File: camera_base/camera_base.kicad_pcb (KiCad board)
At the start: 2 copper layers, 80 x 80 mm, 15 parts, among them J1 Raspberry_Pi_4, J2 Conn_02x06_Odd_Even, SW1 SW_Push_Dual, SW2 SW_Push_Dual, SW3 SW_Push_Dual, SW4 SW_Push_Dual, SW5 SW_Push_Dual

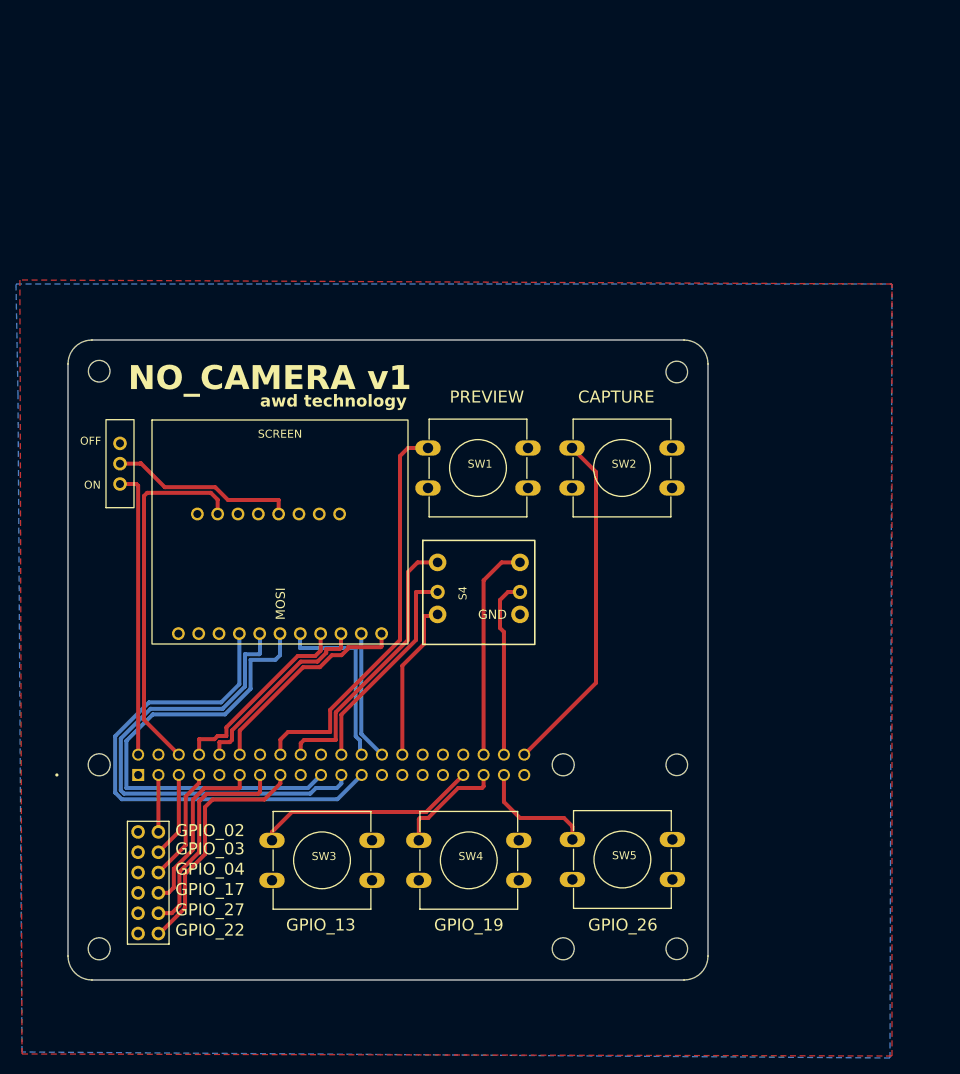
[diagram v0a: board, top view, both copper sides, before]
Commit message: update
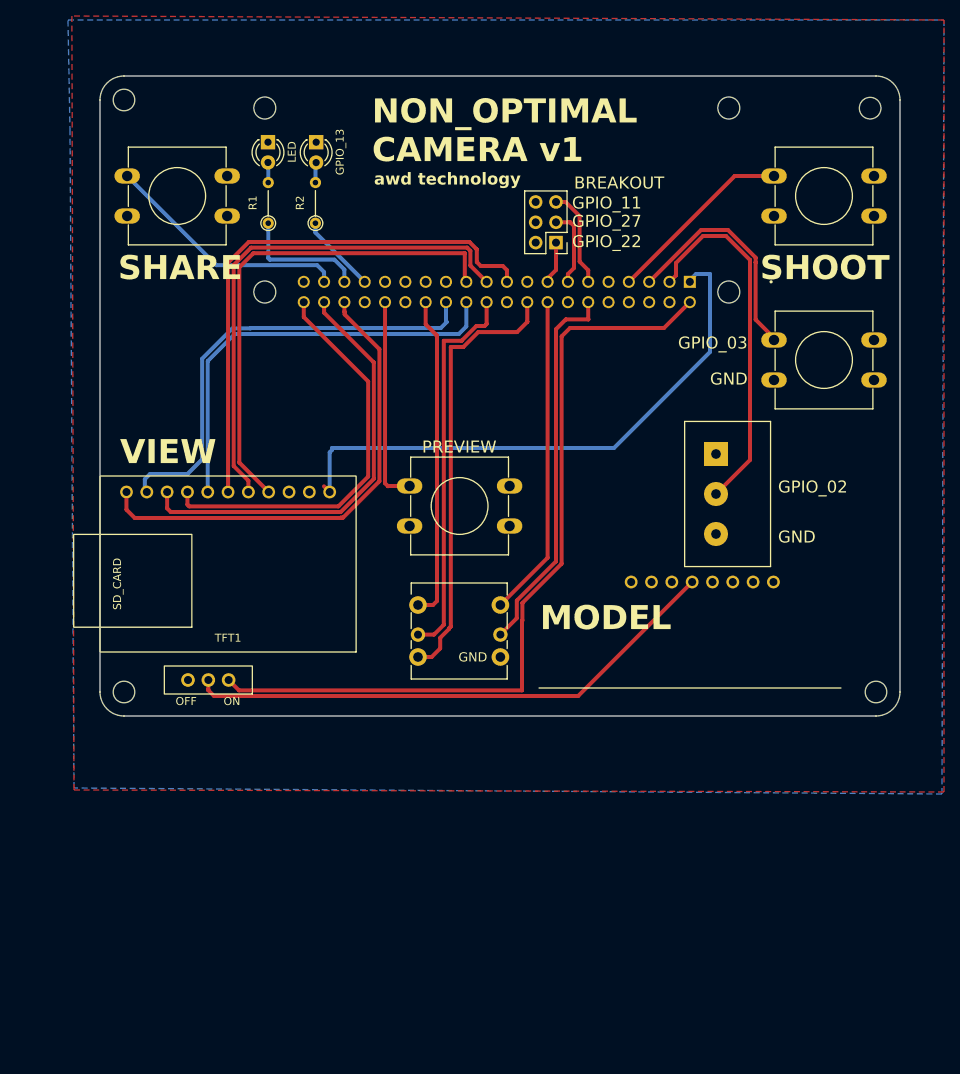
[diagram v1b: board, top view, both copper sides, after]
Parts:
- removed SW4: SW_Push_Dual, camera_base:PUSH_BUTTON_12mm
- added D1: LED, LED_THT:LED_D3.0mm, F.Cu at (81.0, 68.3)
- added D2: LED, LED_THT:LED_D3.0mm, F.Cu at (87.0, 68.3)
- added R1: R, Resistor_THT:R_Axial_DIN0204_L3.6mm_D1.6mm_P5.08mm_Vertical, F.Cu at (81.0, 78.4)
- added R2: R, Resistor_THT:R_Axial_DIN0204_L3.6mm_D1.6mm_P5.08mm_Vertical, F.Cu at (86.9, 78.4)
- added RV1: R_Potentiometer_US, Potentiometer_THT:Potentiometer_Alps_RK163_Single_Horizontal, F.Cu at (137.0, 107.2)
- J2: value Conn_02x06_Odd_Even -> Conn_02x03_Odd_Even; footprint Connector_PinSocket_2.54mm:PinSocket_2x06_P2.54mm_Vertical -> Connector_PinHeader_2.54mm:PinHeader_2x03_P2.54mm_Vertical
- POW1: renamed from LIPO RIDER
- moved SW5 99.9 mm to (69.9, 75.0)
- moved J2 88.9 mm to (117.0, 80.8), turned to 180 degrees
- moved SW3 88.6 mm to (150.8, 95.5)
- moved J1 84.7 mm to (109.6, 75.5), turned to 180 degrees
- moved H3 69.7 mm to (63.0, 137.0)
- moved POW1 63.3 mm to (139.1, 112.2), turned to 180 degrees
- moved SW2 42.4 mm to (150.8, 75.0)
- moved H2 40.9 mm to (156.3, 64.0)
- moved H4 40.6 mm to (157.0, 137.0)
- moved H1 34.0 mm to (63.0, 63.0)
- moved U1 29.2 mm to (73.5, 135.5), turned to 180 degrees
- moved TFT1 6.57 mm to (76.0, 118.0), turned to 180 degrees
- moved S4 5.86 mm to (104.9, 129.4)
- moved SW1 5.28 mm to (105.2, 113.8)
- renumbered SCREEN to TFT1
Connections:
- J1 pad 1: /3v3 -> 3v3
- J1 pad 11: Net-(J1-GPIO17/SPI1_~{CE1}) -> GPIO_11
- J1 pad 13: Net-(J1-GPIO27/SDIO_DAT3) -> GPIO_27
- J1 pad 15: Net-(J1-GPIO22/SDIO_CLK) -> GPIO_22
- J1 pad 17: unconnected-(J1-3V3-Pad17) -> 3v3
- J1 pad 25: unconnected-(J1-GND-Pad25)_1 -> GND
- J1 pad 3: Net-(J1-SDA_I2C1/GPIO02) -> GPIO_02
- J1 pad 32: unconnected-(J1-GPIO12/PWM0-Pad32) -> GPIO_12
- J1 pad 5: Net-(J1-SCL_I2C1/GPIO03) -> GPIO_03
- J1 pad 7: Net-(J1-GPCLK0/GPIO04) -> GPIO_04
- J1 pad 8: GPIO_14 -> unconnected-(J1-GPIO14/UART_TXD-Pad8)
- J1 pad 9: unconnected-(J1-GND-Pad25) -> GND
- J2 pad 1: Net-(J1-SDA_I2C1/GPIO02) -> GPIO_22
- J2 pad 3: Net-(J1-SCL_I2C1/GPIO03) -> GPIO_27
- J2 pad 5: Net-(J1-GPCLK0/GPIO04) -> GPIO_11
- S4 pad 1: GPIO_24 -> GPIO_01
- S4 pad 3: GPIO_01 -> GPIO_24
- S4 pad 5: GPIO_20 -> GPIO_18
- S4 pad 6: GPIO_16 -> GPIO_23
- SW1 pad 1: GPIO_23 -> GPIO_12
- SW2 pad 1: GPIO_21 -> GPIO_04
- SW3 pad 1: GPIO_13 -> GPIO_03
- TFT1 pad 1: /3v3 -> 3v3
- TFT1 pad 11: GPIO_18 -> GPIO_16
- TFT1 pad 8: GPIO_14 -> GPIO_21
- TFT1 pad 9: GPIO_15 -> GPIO_20
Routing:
- net 3v3: track 0.00 -> 72.3 mm
- net Net-(U1-NO): track 36.0 -> 101.3 mm
- net GND: track 45.7 -> 0.00 mm
- net GPIO_02: track 0.00 -> 45.6 mm
- net Net-(POW1-5V): track 23.5 -> 68.0 mm
- net CE1: track 16.2 -> 57.6 mm
- net GPIO_16: track 27.3 -> 60.4 mm
- net GPIO_20: track 22.4 -> 54.5 mm
- net CE0: track 22.4 -> 53.5 mm
- net Net-(J1-GPIO22/SDIO_CLK): track 30.8 -> 0.00 mm
- net GPIO_03: track 0.00 -> 28.8 mm
- net Net-(J1-GPIO27/SDIO_DAT3): track 27.3 -> 0.00 mm
- net GPIO_12: track 0.00 -> 25.9 mm
- net GPIO_15: track 24.5 -> 0.00 mm
- net GPIO_14: track 24.5 -> 0.00 mm
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- added copper zone on F.Cu, net 3v3
- removed copper zone on F.Cu, net /3v3
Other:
- board size 80 x 80 mm -> 100 x 80 mm
- board text added: "BREAKOUT"
- board text added: "GND"
- board text added: "GPIO_11"
- board text added: "MODEL"
- board text added: "NON_OPTIMAL CAMERA v1"
- board text added: "SHARE"
- board text added: "SHOOT"
- board text added: "VIEW"
- board text removed: "CAPTURE"
- board text removed: "GPIO_04"
- board text removed: "GPIO_17"
- board text removed: "GPIO_19"
- board text removed: "GPIO_26"
- board text removed: "MOSI"
- board text removed: "NO_CAMERA v1"
